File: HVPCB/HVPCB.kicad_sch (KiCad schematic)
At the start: 53 parts, among them J1 Micro Fit 10p, Q1 OnSemi FDB12N50TM, U1 NE555DR_C695838, U14 Micro Fit 2P, U16 Micro Fit 2P, U2 SN74LVC1GU04DBVR, U3 PDSE1-S5-D5-M-TR, U4 LM392MX, U5 AO3400A, U6 AO3400A, U7 KT-0603R, U8 KT-0603R, U9 KT-0603R

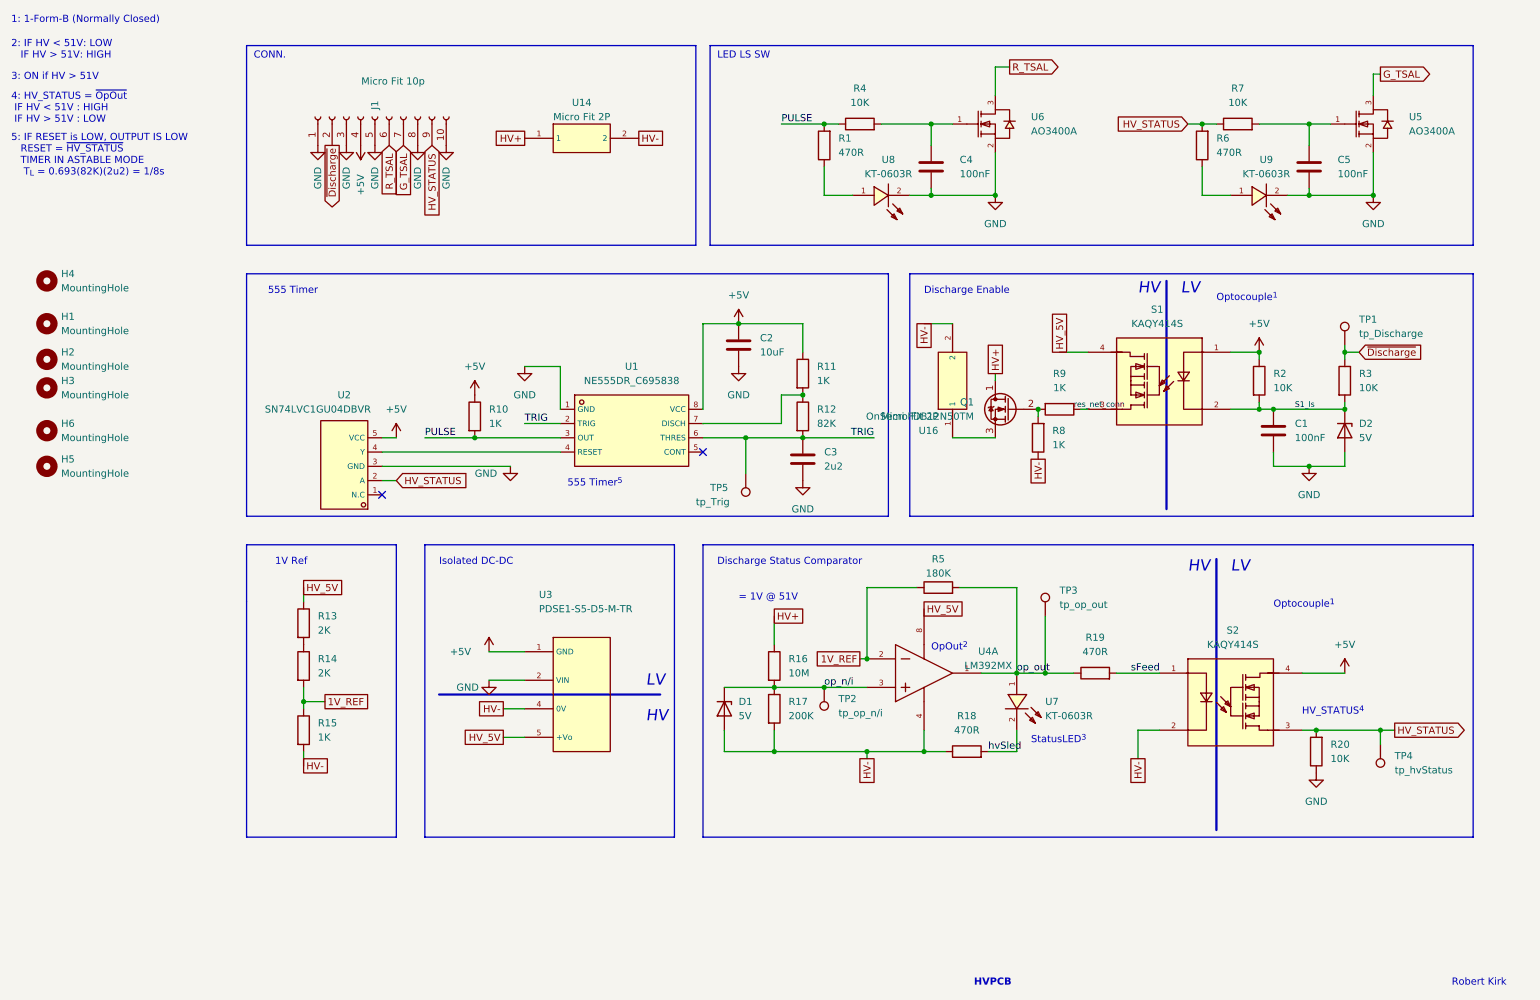
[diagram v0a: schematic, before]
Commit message: HVPCB updates & assembly files
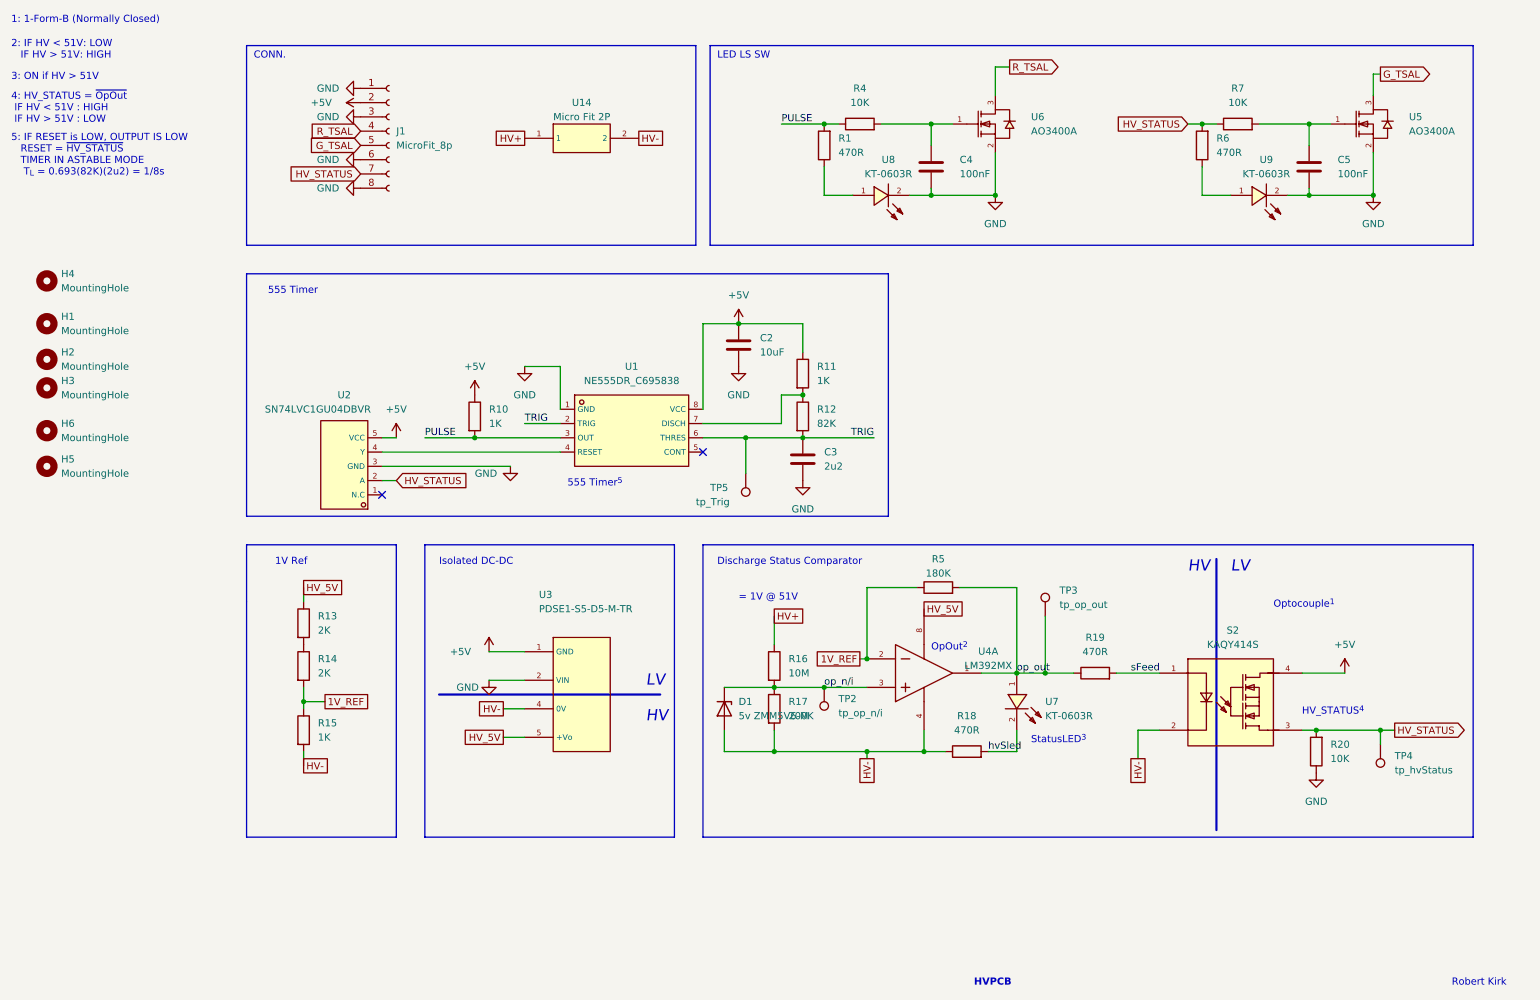
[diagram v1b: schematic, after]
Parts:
- removed C1: 100nF, Resistor_SMD:R_0603_1608Metric_Pad0.98x0.95mm_HandSolder, symbol Device:C
- removed D2: 5V, footprint:LL-34_L3.5-W1.5-RD, symbol Device:D_Zener
- removed J1: Micro Fit 10p, Connector_Molex:Molex_Micro-Fit_3.0_43650-1000_1x10_P3.00mm_Horizontal, symbol Connector:Conn_01x10_Female
- removed Q1: OnSemi FDB12N50TM, Package_TO_SOT_SMD:TO-263-2_TabPin1_D2PAK, symbol Transistor_FET:BS170
- removed R2, R3: 10K, Resistor_SMD:R_0603_1608Metric_Pad0.98x0.95mm_HandSolder, symbol Device:R
- removed R8, R9: 1K, Resistor_SMD:R_0603_1608Metric_Pad0.98x0.95mm_HandSolder, symbol Device:R
- removed S1: KAQY414S, footprint:SOP-4_L3.9-W4.4-P2.54-LS7.0-BR, symbol default_lib:KAQY414S
- removed TP1: tp_Discharge, TestPoint:TestPoint_THTPad_D2.0mm_Drill1.0mm, symbol Connector:TestPoint
- removed U16: Micro Fit 2P, footprint:CONN-TH_43045-0200, symbol default_lib:0430450200
- added J1: MicroFit_8p, Connector_Molex:Molex_Micro-Fit_3.0_43650-0800_1x08_P3.00mm_Horizontal, symbol Connector:Conn_01x08_Female
- C2, C3, C4, C5: footprint Resistor_SMD:R_0603_1608Metric_Pad0.98x0.95mm_HandSolder -> Capacitor_SMD:C_0603_1608Metric_Pad1.08x0.95mm_HandSolder
- D1: value 5V -> 5v ZMM5V6-M; footprint footprint:LL-34_L3.5-W1.5-RD -> Diode_SMD:D_MiniMELF
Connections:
- net +5V: now also J1.2 (Pin_2)
- net GND: now also J1.1 (Pin_1), J1.3 (Pin_3), J1.6 (Pin_6), J1.8 (Pin_8)
- net G_TSAL: now also J1.5 (Pin_5)
- net HV_STATUS: now also J1.7 (Pin_7)
- net R_TSAL: now also J1.4 (Pin_4)
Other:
- note removed: "Discharge Enable"
